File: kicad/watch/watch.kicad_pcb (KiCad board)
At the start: 2 copper layers, 35.6 x 25.4 mm, 53 parts, among them IC1 113990582, J1 Conn_01x04_Female, J2 Conn_01x04_Female, J3 Conn_01x04_Female, J4 Memory LCD, J5 LCD Frontlight, J6 Buzzer, Q1 DMN6140L, Q2 DMN6140L, U1 W25X20CLUXIG, U2 MCP73831-2-OT, U3 M41T62Q, U4 TPS63001, Y1 Crystal, Y2 32.768 kHz

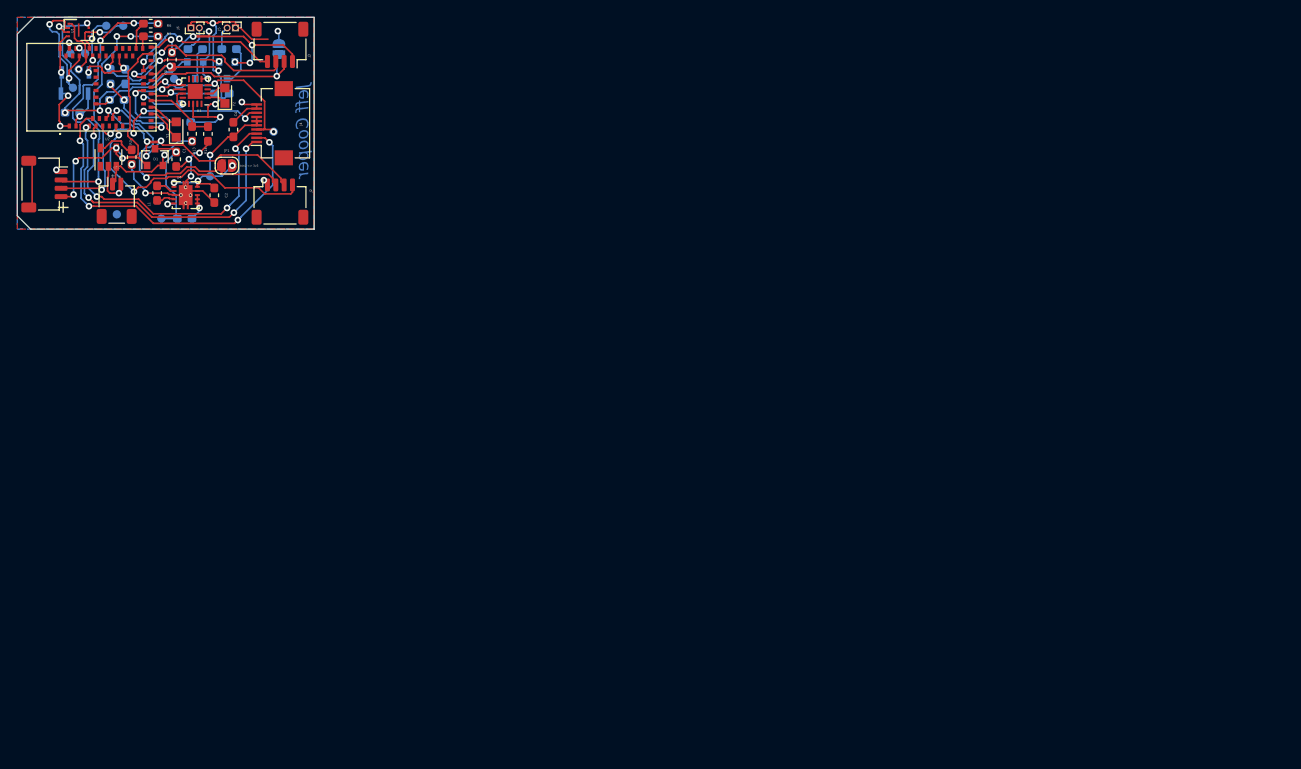
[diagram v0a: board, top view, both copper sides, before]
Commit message: checkpoint
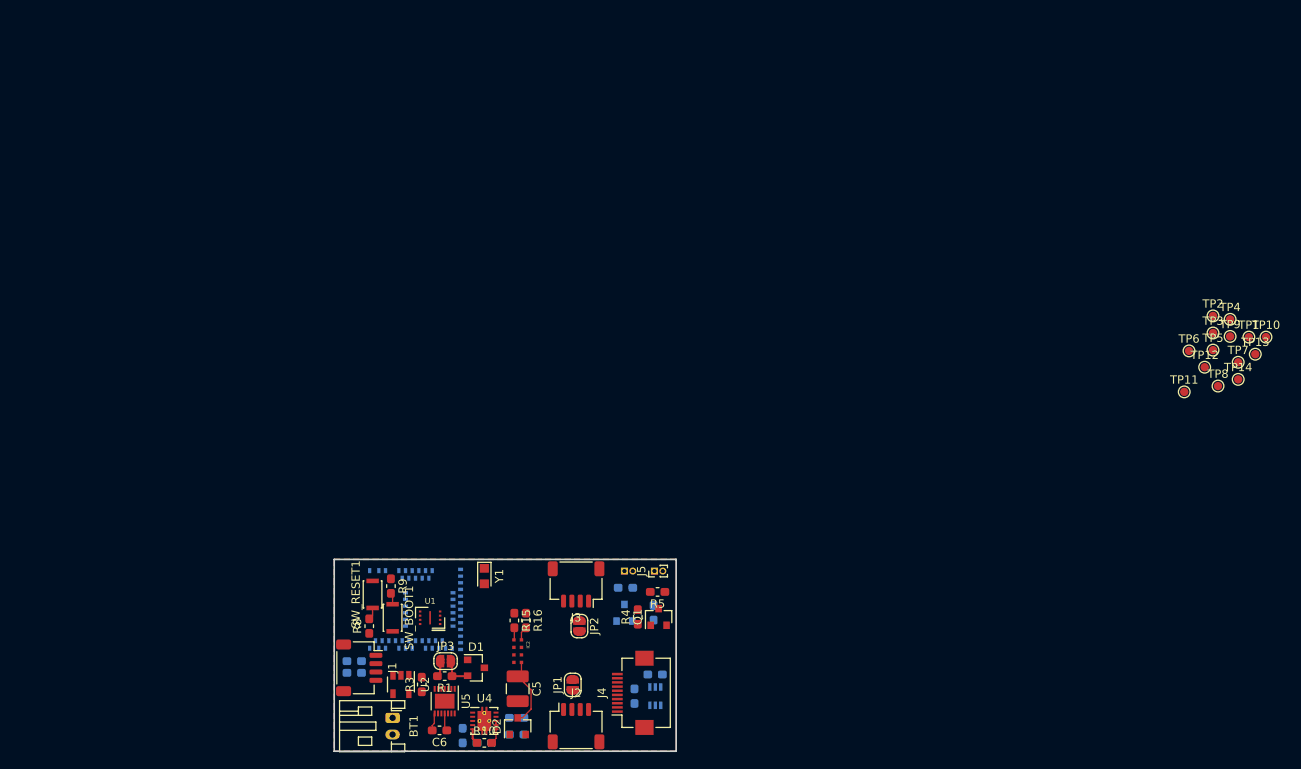
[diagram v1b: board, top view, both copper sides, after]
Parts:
- removed R13: 2M, Resistor_SMD:R_0603_1608Metric_Pad1.05x0.95mm_HandSolder
- removed R14: 4M, Resistor_SMD:R_0603_1608Metric_Pad1.05x0.95mm_HandSolder
- removed Y2: 32.768 kHz, Crystal:Crystal_SMD_2012-2Pin_2.0x1.2mm_HandSoldering
- added C5: 11mF, Capacitor_SMD:C_1210_3225Metric_Pad1.42x2.65mm_HandSolder, F.Cu at (60.0, 80.5)
- added C6: 4.7 uF, Capacitor_SMD:C_0603_1608Metric_Pad1.05x0.95mm_HandSolder, F.Cu at (50.6, 85.5)
- added D2: D_Schottky, Diode_SMD:D_SOT-23_ANK, F.Cu at (60.0, 85.0)
- added IC2: M41T62LC6F, libs:LCC90P230X50X80-8N, F.Cu at (60.0, 76.0)
- added JP3: Jumper_NO_Small, Jumper:SolderJumper-2_P1.3mm_Open_RoundedPad1.0x1.5mm, F.Cu at (51.4, 77.2)
- added L2: 4.7 uH, Inductor_SMD:L_0603_1608Metric_Pad1.05x0.95mm_HandSolder, B.Cu at (76.5, 78.8)
- added R1: 10 m, Resistor_SMD:R_0603_1608Metric_Pad1.05x0.95mm_HandSolder, F.Cu at (51.2, 79.0)
- added TP14: TestPoint, TestPoint:TestPoint_Pad_D1.0mm, F.Cu at (146.4, 43.4)
- added U5: MAX17260, Package_DFN_QFN:DFN-14-1EP_3x3mm_P0.4mm_EP1.78x2.35mm, F.Cu at (51.2, 82.0)
- BT1: footprint Connector_JST:JST_SH_SM02B-SRSS-TB_1x02-1MP_P1.00mm_Horizontal -> Connector_JST:JST_PH_S2B-PH-K_1x02_P2.00mm_Horizontal
- C1, C2, C3, C4, IC1, J6, R6, R7: moved to B.Cu
- JP2, Q1, R10, R15, R16, R4, R5, R8, R9, SW_BOOT1, SW_RESET1, TP1, TP10, TP11, TP12, TP13, TP2, TP3, TP4, TP5, TP6, TP7, TP8, TP9: moved to F.Cu
- L1: value 1uF -> 2.2uH; moved to B.Cu
- U3: value M41T62Q -> TPS61222DCK; footprint Package_DFN_QFN:VQFN-16-1EP_3x3mm_P0.5mm_EP1.8x1.8mm -> Package_TO_SOT_SMD:Texas_R-PDSO-G6; moved to B.Cu
- moved TP10 142.0 mm to (149.7, 38.3)
- moved TP3 141.1 mm to (143.4, 37.9)
- moved TP4 141.0 mm to (145.4, 36.2)
- moved TP9 139.8 mm to (145.4, 38.3)
- moved TP12 139.8 mm to (142.4, 42.0)
- moved TP11 138.1 mm to (139.9, 44.9)
- moved TP13 132.2 mm to (148.4, 40.4)
- moved TP2 132.0 mm to (143.4, 35.8)
- moved TP8 128.9 mm to (144.0, 44.2)
- moved TP1 126.0 mm to (147.7, 38.3)
- moved TP6 126.0 mm to (140.5, 40.0)
- moved TP5 125.9 mm to (143.4, 39.9)
- moved TP7 118.9 mm to (146.4, 41.4)
- moved U3 91.1 mm to (76.5, 81.4), turned to 90 degrees
- moved R4 90.5 mm to (74.4, 71.9)
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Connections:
- D1 pad 2: +BATT -> BATTPOW
- IC1 pad 20: BATREAD -> (no net)
- J4 pad 5: +3V3 -> +5V
- J4 pad 6: +3V3 -> +5V
- J4 pad 7: +3V3 -> +5V
- U3 pad 1: Net-(U3-Pad1) -> VIN
- U3 pad 2: Net-(U3-Pad2) -> +5V
- U3 pad 3: (no net) -> GND
- U3 pad 4: SQW -> +5V
- U3 pad 5: GND -> Net-(L2-Pad2)
- U3 pad 6: (no net) -> VIN
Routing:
- net +3V3: track 102.3 -> 0.00 mm, vias 14 -> 0
- net GND: track 95.2 -> 2.14 mm, vias 23 -> 0
- net LCD_MOSI: track 44.1 -> 0.00 mm, vias 4 -> 0
- net LCD_CLK: track 37.9 -> 0.00 mm, vias 4 -> 0
- net LCD_CS: track 37.5 -> 0.00 mm, vias 4 -> 0
- net VBUS: track 34.3 -> 0.00 mm, vias 4 -> 0
- net USB_DP: track 34.0 -> 0.00 mm, vias 4 -> 0
- net BTN3: track 32.7 -> 0.00 mm, vias 4 -> 0
- net BTN1: track 31.9 -> 0.00 mm, vias 2 -> 0
- net BTN2: track 31.1 -> 0.00 mm, vias 2 -> 0
- net USB_DN: track 30.2 -> 0.00 mm, vias 4 -> 0
- net SQW: track 23.0 -> 0.00 mm, vias 3 -> 0
- net BTN5: track 22.6 -> 0.00 mm, vias 2 -> 0
- net EXTMODE: track 22.4 -> 0.00 mm, vias 4 -> 0
- net BTN6: track 20.5 -> 0.00 mm, vias 1 -> 0
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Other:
- board size 35.6 x 25.4 mm -> 41 x 23 mm
- net class Default: clearance 0.2 -> 0.14; trace_width 0.2 -> 0.15; via_dia 0.8 -> 0.5; via_drill 0.4 -> 0.3
- net class power added: clearance 0.2, trace_width 0.25, via_dia 0.8, via_drill 0.4
- rule pad_to_mask_clearance: 0.2 -> 0
- rule trace_clearance: 0.2 -> 0.14
- rule trace_min: 0.2 -> 0.13
- rule via_min_drill: 0.3 -> 0.2
- rule via_min_size: 0.4 -> 0.45
- board text removed: "+"
- board text removed: "+ -"
- board text removed: "Jeff Cooper"
- board text removed: "btn2 <> 3v3"
- board text removed: "jeff@thejeffcooper.com Proudly designed in Pittsburgh, PA"
- board text removed: "nrf52 watch mk 1 rev 1"
